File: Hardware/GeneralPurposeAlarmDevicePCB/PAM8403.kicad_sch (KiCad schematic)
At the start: 2 parts

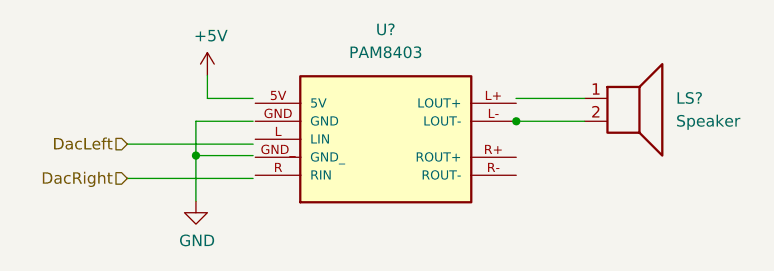
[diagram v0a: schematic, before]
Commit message: updated PCB
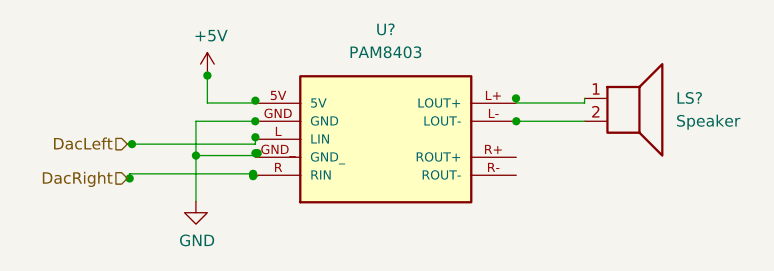
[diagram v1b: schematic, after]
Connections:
- net GND: now also U?.GND
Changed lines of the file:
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@@
 (kicad_sch (version 20211123) (generator eeschema)
   (paper "A4")
+  (junction (at 132.588 93.726) (diameter 0) (color 0 0 0 0)
+  )
+  (junction (at 118.364 96.52) (diameter 0) (color 0 0 0 0)
+  )
   (junction (at 125.73 93.98) (diameter 0) (color 0 0 0 0)
+  )
+  (junction (at 132.334 93.726) (diameter 0) (color 0 0 0 0)
+  )
+  (junction (at 132.08 96.012) (diameter 0) (color 0 0 0 0)
+  )
+  (junction (at 161.29 87.63) (diameter 0) (color 0 0 0 0)
+  )
+  (junction (at 132.334 87.884) (diameter 0) (color 0 0 0 0)
+  )
+  (junction (at 132.334 91.948) (diameter 0) (color 0 0 0 0)
+  )
+  (junction (at 118.618 92.71) (diameter 0) (color 0 0 0 0)
+  )
+  (junction (at 127 85.09) (diameter 0) (color 0 0 0 0)
+  )
+  (junction (at 132.32 90.17) (diameter 0) (color 0 0 0 0)
   )
   (junction (at 161.32 90.17) (diameter 0) (color 0 0 0 0)
   )
-  (wire (pts (xy 127 87.63) (xy 127 85.09))
+  (junction (at 132.08 96.266) (diameter 0) (color 0 0 0 0)
+  )
+  (wire (pts (xy 127 88.138) (xy 132.334 88.138))
     (stroke (width 0) (type default) (color 0 0 0 0))
   )
-  (wire (pts (xy 125.73 93.98) (xy 132.08 93.98))
+  (wire (pts (xy 125.73 93.98) (xy 132.588 93.98))
     (stroke (width 0) (type default) (color 0 0 0 0))
   )
-  (wire (pts (xy 132.08 90.17) (xy 125.73 90.17))
+  (wire (pts (xy 118.364 96.52) (xy 118.364 96.774))
     (stroke (width 0) (type default) (color 0 0 0 0))
   )
-  (wire (pts (xy 118.11 92.71) (xy 132.08 92.71))
+  (wire (pts (xy 118.618 92.456) (xy 118.618 92.71))
+    (stroke (width 0) (type default) (color 0 0 0 0))
+  )
+  (wire (pts (xy 132.08 91.948) (xy 132.08 92.202))
+    (stroke (width 0) (type default) (color 0 0 0 0))
+  )
+  (wire (pts (xy 132.334 87.884) (xy 132.588 87.884))
+    (stroke (width 0) (type default) (color 0 0 0 0))
+  )
+  (wire (pts (xy 161.29 88.138) (xy 168.91 88.138))
+    (stroke (width 0) (type default) (color 0 0 0 0))
+  )
+  (wire (pts (xy 118.364 96.012) (xy 118.364 96.52))
+    (stroke (width 0) (type default) (color 0 0 0 0))
+  )
+  (wire (pts (xy 118.618 92.71) (xy 132.334 92.71))
+    (stroke (width 0) (type default) (color 0 0 0 0))
+  )
+  (wire (pts (xy 132.334 90.17) (xy 132.32 90.17))
+    (stroke (width 0) (type default) (color 0 0 0 0))
+  )
+  (wire (pts (xy 132.334 92.71) (xy 132.334 91.948))
+    (stroke (width 0) (type default) (color 0 0 0 0))
+  )
+  (wire (pts (xy 132.08 96.266) (xy 132.08 96.012))
+    (stroke (width 0) (type default) (color 0 0 0 0))
+  )
+  (wire (pts (xy 161.036 87.63) (xy 161.29 87.63))
+    (stroke (width 0) (type default) (color 0 0 0 0))
+  )
+  (wire (pts (xy 168.91 88.138) (xy 168.91 87.63))
+    (stroke (width 0) (type default) (color 0 0 0 0))
+  )
+  (wire (pts (xy 125.73 90.17) (xy 125.73 93.98))
+    (stroke (width 0) (type default) (color 0 0 0 0))
+  )
+  (wire (pts (xy 127 88.138) (xy 127 85.09))
+    (stroke (width 0) (type default) (color 0 0 0 0))
+  )
+  (wire (pts (xy 132.08 93.726) (xy 132.334 93.726))
+    (stroke (width 0) (type default) (color 0 0 0 0))
+  )
+  (wire (pts (xy 132.08 96.012) (xy 132.334 96.012))
     (stroke (width 0) (type default) (color 0 0 0 0))
   )
@@
     (stroke (width 0) (type default) (color 0 0 0 0))
   )
+  (wire (pts (xy 118.364 96.012) (xy 132.08 96.012))
+    (stroke (width 0) (type default) (color 0 0 0 0))
+  )
+  (wire (pts (xy 132.08 96.52) (xy 132.08 96.266))
+    (stroke (width 0) (type default) (color 0 0 0 0))
+  )
   (wire (pts (xy 161.29 90.17) (xy 161.32 90.17))
     (stroke (width 0) (type default) (color 0 0 0 0))
   )
-  (wire (pts (xy 118.11 96.52) (xy 132.08 96.52))
+  (wire (pts (xy 161.29 87.63) (xy 161.29 87.884))
     (stroke (width 0) (type default) (color 0 0 0 0))
   )
-  (wire (pts (xy 125.73 90.17) (xy 125.73 93.98))
+  (wire (pts (xy 127 85.09) (xy 127.254 85.09))
     (stroke (width 0) (type default) (color 0 0 0 0))
   )
-  (wire (pts (xy 127 87.63) (xy 132.08 87.63))
+  (wire (pts (xy 132.334 93.726) (xy 132.588 93.726))
     (stroke (width 0) (type default) (color 0 0 0 0))
   )
-  (wire (pts (xy 161.29 87.63) (xy 168.91 87.63))
+  (wire (pts (xy 132.334 91.948) (xy 132.08 91.948))
+    (stroke (width 0) (type default) (color 0 0 0 0))
+  )
+  (wire (pts (xy 161.036 87.63) (xy 161.036 87.884))
+    (stroke (width 0) (type default) (color 0 0 0 0))
+  )
+  (wire (pts (xy 132.08 96.266) (xy 132.588 96.266))
+    (stroke (width 0) (type default) (color 0 0 0 0))
+  )
+  (wire (pts (xy 118.364 96.774) (xy 118.11 96.774))
+    (stroke (width 0) (type default) (color 0 0 0 0))
+  )
+  (wire (pts (xy 132.334 93.472) (xy 132.334 93.726))
     (stroke (width 0) (type default) (color 0 0 0 0))
   )
@@
     (stroke (width 0) (type default) (color 0 0 0 0))
   )
+  (wire (pts (xy 118.364 92.71) (xy 118.618 92.71))
+    (stroke (width 0) (type default) (color 0 0 0 0))
+  )
+  (wire (pts (xy 132.32 90.17) (xy 125.73 90.17))
+    (stroke (width 0) (type default) (color 0 0 0 0))
+  )
